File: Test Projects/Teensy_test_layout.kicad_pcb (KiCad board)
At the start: 2 copper layers, 254 x 127 mm, 309 parts, among them P1 CONN_01X02, P10 CONN_01X06, P11 CONN_01X06, P12 CONN_01X06, P13 CONN_01X08, P14 CONN_01X08, P15 CONN_01X08, P16 CONN_01X08, P17 CONN_01X08, P18 CONN_01X08, P19 CONN_01X08, P2 CONN_01X03, P20 CONN_01X08, P21 CONN_01X07, P22 CONN_01X08, P23 CONN_01X08, P24 CONN_01X08, P25 CONN_01X08, P26 CONN_01X08, P27 CONN_01X08, P28 CONN_01X08, P29 CONN_01X08, P3 COLS0, P30 CONN_01X03, P31 PIN20, P32 PIN8, P33 SIO2, P34 ~HOLD~/SIO3, P35 PIN37, P36 PIN29, P37 PIN31, P38 CONN_01X06, P39 CONN_01X06, P4 COLS1, P40 CONN_01X08, P41 CONN_01X08, P42 CONN_01X08, P43 CONN_01X08, P44 CONN_01X08, P45 CONN_01X08, P46 CONN_01X08, P47 CONN_01X08, P48 CONN_01X08, P49 CONN_01X08, P5 CONN_01X06, P50 CONN_01X08, P51 CONN_01X08, P52 CONN_01X08, P53 CONN_01X08, P54 CONN_01X08, P55 CONN_01X08, P56 CONN_01X01, P57 CONN_01X01, P58 VUU, P59 CONN_01X01, P6 CONN_01X06, P60 CONN_01X01, P61 CONN_01X01, P62 UGND, P63 CONN_01X01, P64 DIN1, P65 DOUT1, P66 SDA0, P67 SCL0, P68 MCLK, P69 BCLK, P7 CONN_01X06, P70 LRCLK, P71 DIN0, P72 DOUT0, P73 IN2TTL, P74 CONN_01X08, P75 CONN_01X08, P76 CONN_01X08, P77 CONN_01X08, P78 CONN_01X08, P79 CONN_01X08, P8 CONN_01X06, P80 CONN_01X08, P81 CONN_01X08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

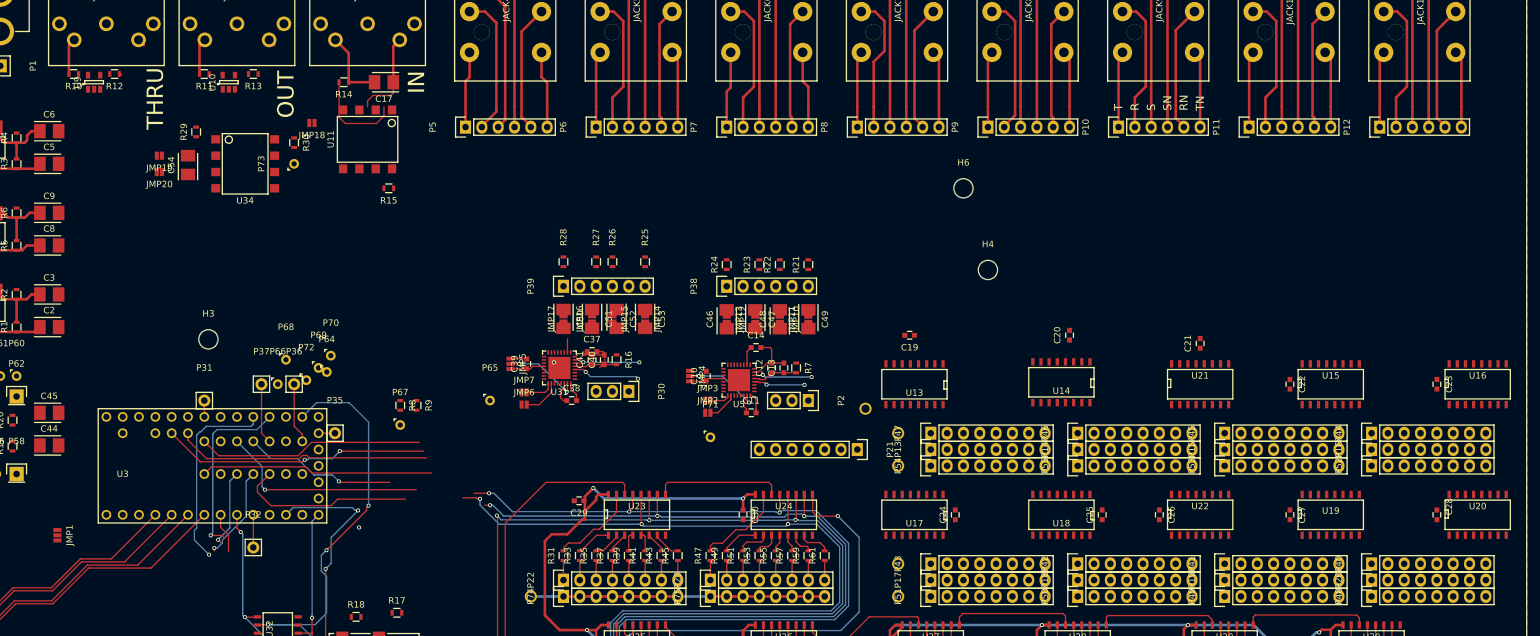
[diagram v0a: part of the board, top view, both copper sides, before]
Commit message: more layout
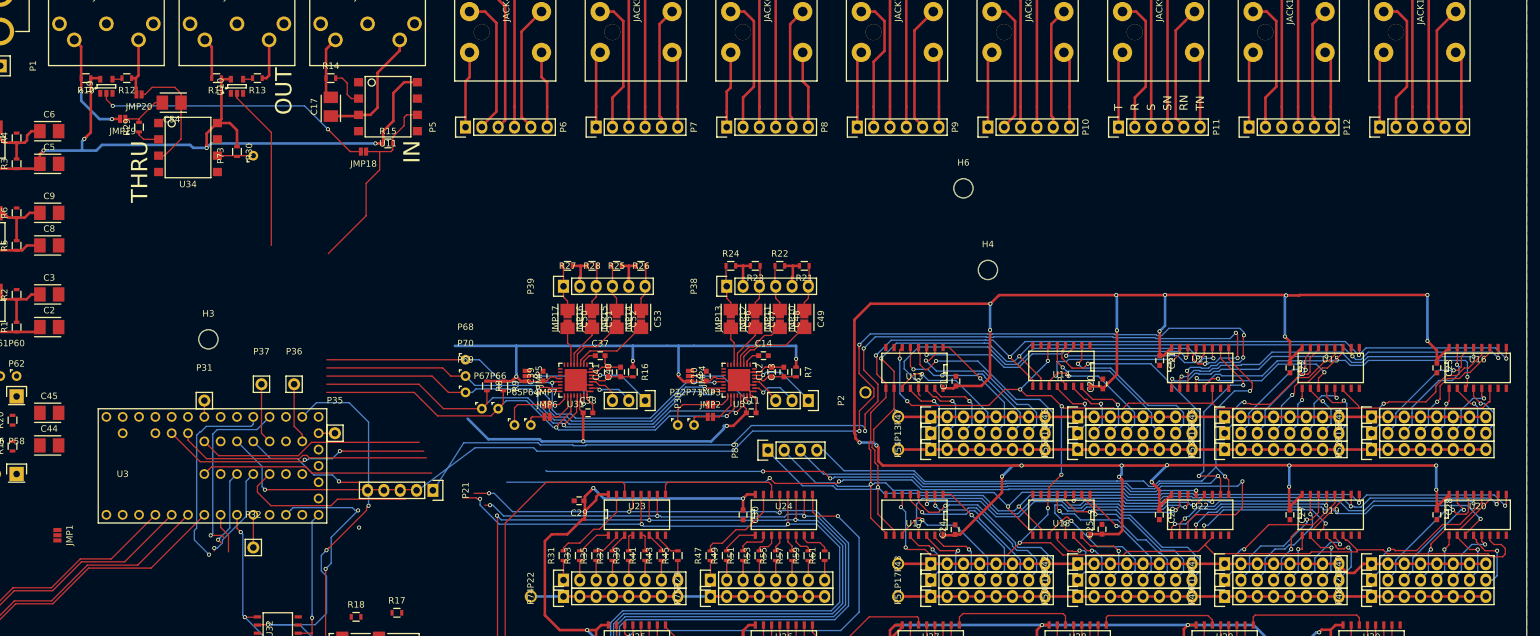
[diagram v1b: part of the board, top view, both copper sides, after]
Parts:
- added P89: CONN_01X04, Pin_Headers:Pin_Header_Straight_1x04, F.Cu at (161.3, 104.2)
- P21: value CONN_01X07 -> CONN_01X05; footprint Pin_Headers:Pin_Header_Straight_1x07 -> Pin_Headers:Pin_Header_Straight_1x05
- moved P21 66.3 mm to (109.2, 110.5)
- moved P72 58.2 mm to (147.3, 100.3)
- moved P66 34.5 mm to (119.4, 97.8)
- moved P64 32.8 mm to (124.5, 100.3)
- moved P68 27.9 mm to (114.3, 90.2)
- moved P69 23.2 mm to (114.3, 95.2)
- moved P70 21.2 mm to (114.3, 92.7)
- moved R8 13.8 mm to (117.6, 94.2)
- moved R9 13.8 mm to (120.2, 94.2)
- moved P67 13.0 mm to (116.8, 97.8)
- moved JMP20 12.5 mm to (63.5, 48.9)
- moved C19 10.1 mm to (190.6, 93.5), turned to 90 degrees
- moved C54 10.0 mm to (68.6, 50.2), turned to 180 degrees
- moved U34 9.25 mm to (71.1, 57.1)
- moved JMP18 9.18 mm to (98.4, 57.8)
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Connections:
- U21 pad 10: A -> C
- U21 pad 9: B -> D
- U22 pad 10: A -> C
- U22 pad 9: B -> D
- U3 pad 27: KA -> (no net)
- U3 pad 28: KB -> (no net)
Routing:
- net VDD: track 0.00 -> 346.7 mm, vias 0 -> 22
- net B: track 0.00 -> 271.8 mm, vias 0 -> 8
- net A: track 0.00 -> 271.7 mm, vias 0 -> 8
- net EN: track 0.00 -> 260.7 mm, vias 0 -> 10
- net KA1: track 39.7 -> 233.2 mm, vias 0 -> 6
- net VKK: track 0.15 -> 184.3 mm
- net KGND: track 0.15 -> 183.0 mm
- net KA0: track 41.8 -> 202.8 mm, vias 2 -> 7
- net KA3: track 35.2 -> 161.6 mm, vias 0 -> 3
- net KA2: track 36.2 -> 146.4 mm, vias 0 -> 3
- net +5V: track 239.8 -> 341.4 mm, vias 8 -> 12
- net C: track 0.00 -> 99.9 mm, vias 0 -> 3
- net D: track 0.00 -> 94.7 mm, vias 0 -> 2
- net SCL0: track 0.00 -> 80.6 mm, vias 0 -> 2
- net SDA0: track 0.00 -> 80.2 mm, vias 0 -> 2
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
